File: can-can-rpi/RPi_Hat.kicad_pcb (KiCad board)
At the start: 2 copper layers, 65 x 56 mm, 5 parts, among them J2 RPi_GPIO

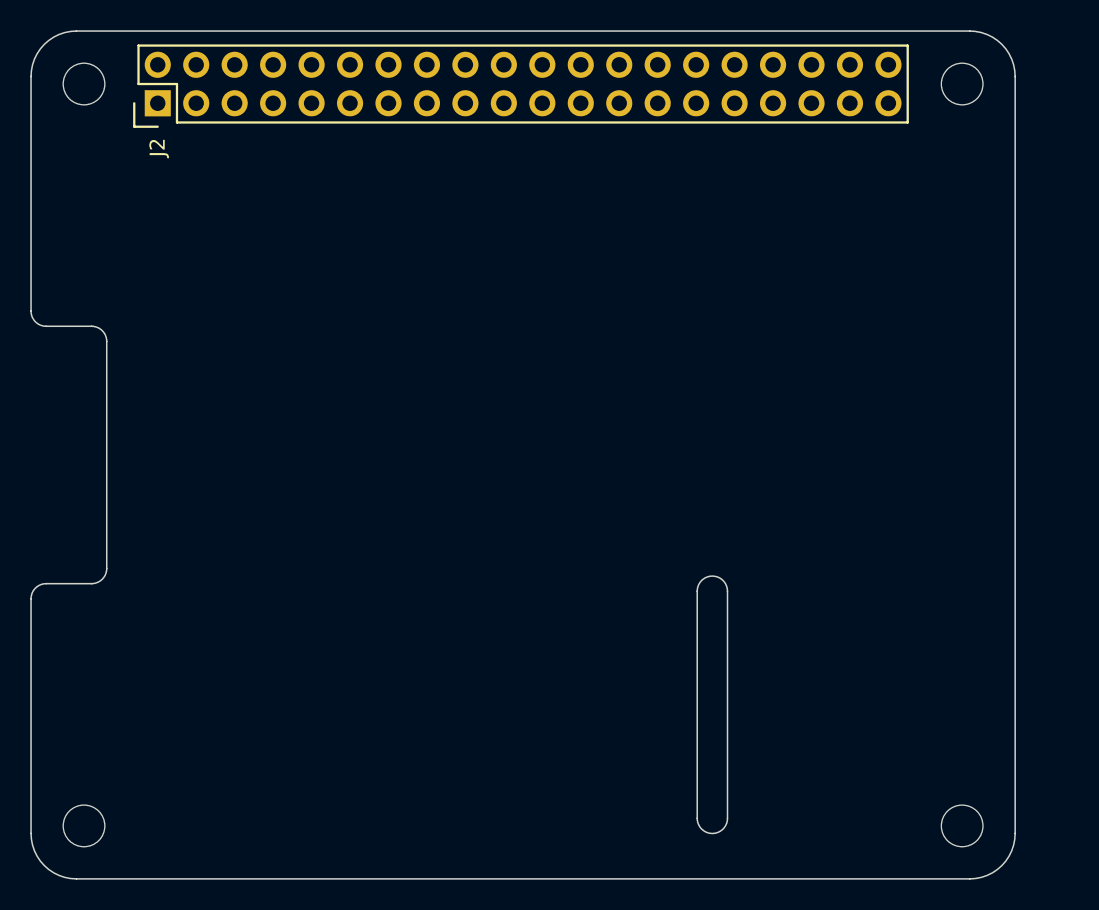
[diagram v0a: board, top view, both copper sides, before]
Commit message: wip
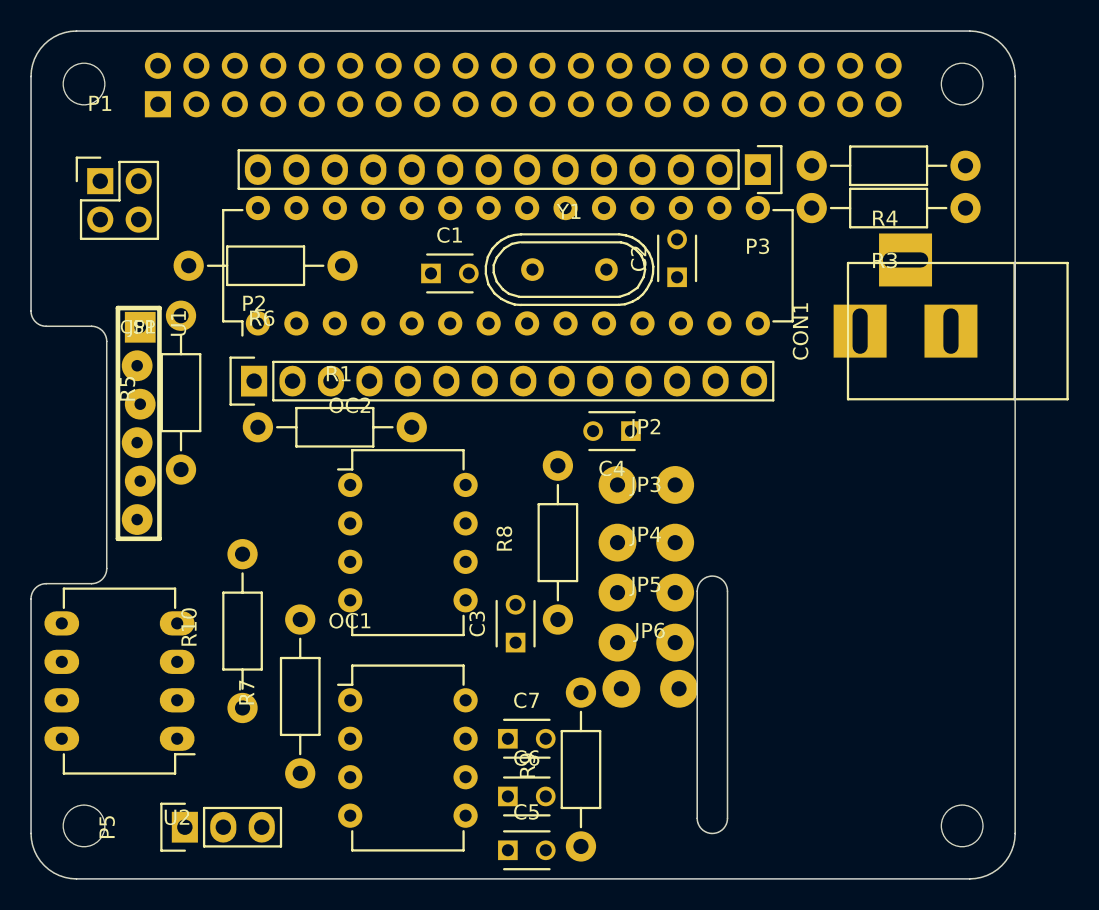
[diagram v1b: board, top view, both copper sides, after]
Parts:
- removed J2: RPi_GPIO, RPi_Hat:Pin_Header_Straight_2x20
- added C1: 100nF, Capacitors_ThroughHole:C_Disc_D3_P2.5, F.Cu at (112.8, 87.6)
- added C2: 100nF, Capacitors_ThroughHole:C_Disc_D3_P2.5, F.Cu at (129.0, 87.9)
- added C3: 27pF, Capacitors_ThroughHole:C_Disc_D3_P2.5, F.Cu at (118.4, 112.0)
- added C4: 27pF, Capacitors_ThroughHole:C_Disc_D3_P2.5, F.Cu at (126.0, 98.0)
- added C5: 100nF, Capacitors_ThroughHole:C_Disc_D3_P2.5, F.Cu at (117.9, 125.7)
- added C6: 100nF, Capacitors_ThroughHole:C_Disc_D3_P2.5, F.Cu at (117.9, 122.2)
- added C7: 100nF, Capacitors_ThroughHole:C_Disc_D3_P2.5, F.Cu at (117.9, 118.4)
- added CON1: BARREL_JACK, Connect:BARREL_JACK, F.Cu at (147.3, 91.4)
- added J1: RPi_GPIO, Socket_Strips:Socket_Strip_Straight_2x20, B.Cu at (94.7, 76.5)
- added JP1: ICSP, ICSP:ICSP, F.Cu at (93.5, 91.2)
- added JP2: JUMPER, Wire_Pads:SolderWirePad_2x_1mmDrill, F.Cu at (127.0, 101.6)
- added JP3: JUMPER, Wire_Pads:SolderWirePad_2x_1mmDrill, F.Cu at (127.0, 105.4)
- added JP4: JUMPER, Wire_Pads:SolderWirePad_2x_1mmDrill, F.Cu at (127.0, 108.7)
- added JP5: JUMPER, Wire_Pads:SolderWirePad_2x_1mmDrill, F.Cu at (127.0, 112.0)
- added JP6: JUMPER, Wire_Pads:SolderWirePad_2x_1mmDrill, F.Cu at (127.3, 115.1)
- added OC1: 6N137, Housings_DIP:DIP-8_W7.62mm, F.Cu at (107.4, 115.8)
- added OC2: 6N137, Housings_DIP:DIP-8_W7.62mm, F.Cu at (107.4, 101.6)
- added P1: CONN_02X02, Pin_Headers:Pin_Header_Straight_2x02, F.Cu at (90.9, 81.5)
- added P2: CONN_01X14, Socket_Strips:Socket_Strip_Straight_1x14, F.Cu at (101.1, 94.7)
- added P3: CONN_01X14, Socket_Strips:Socket_Strip_Straight_1x14, F.Cu at (134.4, 80.8)
- added P5: CONN_01X03, Pin_Headers:Pin_Header_Straight_1x03, F.Cu at (96.5, 124.2)
- added R1: 15k, Resistors_ThroughHole:Resistor_Horizontal_RM10mm, F.Cu at (106.4, 97.8)
- added R10: 390, Resistors_ThroughHole:Resistor_Horizontal_RM10mm, F.Cu at (100.3, 111.3)
- added R3: 3k3, Resistors_ThroughHole:Resistor_Horizontal_RM10mm, F.Cu at (143.0, 83.3)
- added R4: 3k3, Resistors_ThroughHole:Resistor_Horizontal_RM10mm, F.Cu at (143.0, 80.5)
- added R5: 470, Resistors_ThroughHole:Resistor_Horizontal_RM10mm, F.Cu at (96.3, 95.5)
- added R6: 470, Resistors_ThroughHole:Resistor_Horizontal_RM10mm, F.Cu at (101.9, 87.1)
- added R7: 390, Resistors_ThroughHole:Resistor_Horizontal_RM10mm, F.Cu at (104.1, 115.6)
- added R8: 390, Resistors_ThroughHole:Resistor_Horizontal_RM10mm, F.Cu at (121.2, 105.4)
- added R9: 390, Resistors_ThroughHole:Resistor_Horizontal_RM10mm, F.Cu at (122.7, 120.4)
- added U1: PIC18F25K80, Housings_DIP:DIP-28_W7.62mm, F.Cu at (101.3, 90.9)
- added U2: MCP2562-I/P, Housings_DIP:DIP-8_W7.62mm_LongPads, F.Cu at (96.0, 118.4)
- added Y1: 16MHz, Crystals:Crystal_HC49-U_Vertical, F.Cu at (121.9, 87.4)
